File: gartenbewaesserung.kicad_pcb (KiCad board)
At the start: 2 copper layers, 57 x 73.5 mm, 13 parts, among them J1 24VDC IN, J2 Relais, J3 4..20mA Hydrostatischer Sensor, J4 1-Wire A, J5 1-Wire B, J6 ADS1115 Modul, Q1 IRLZ44N, U1 WeMos_D1_mini, U2 ULN2803A

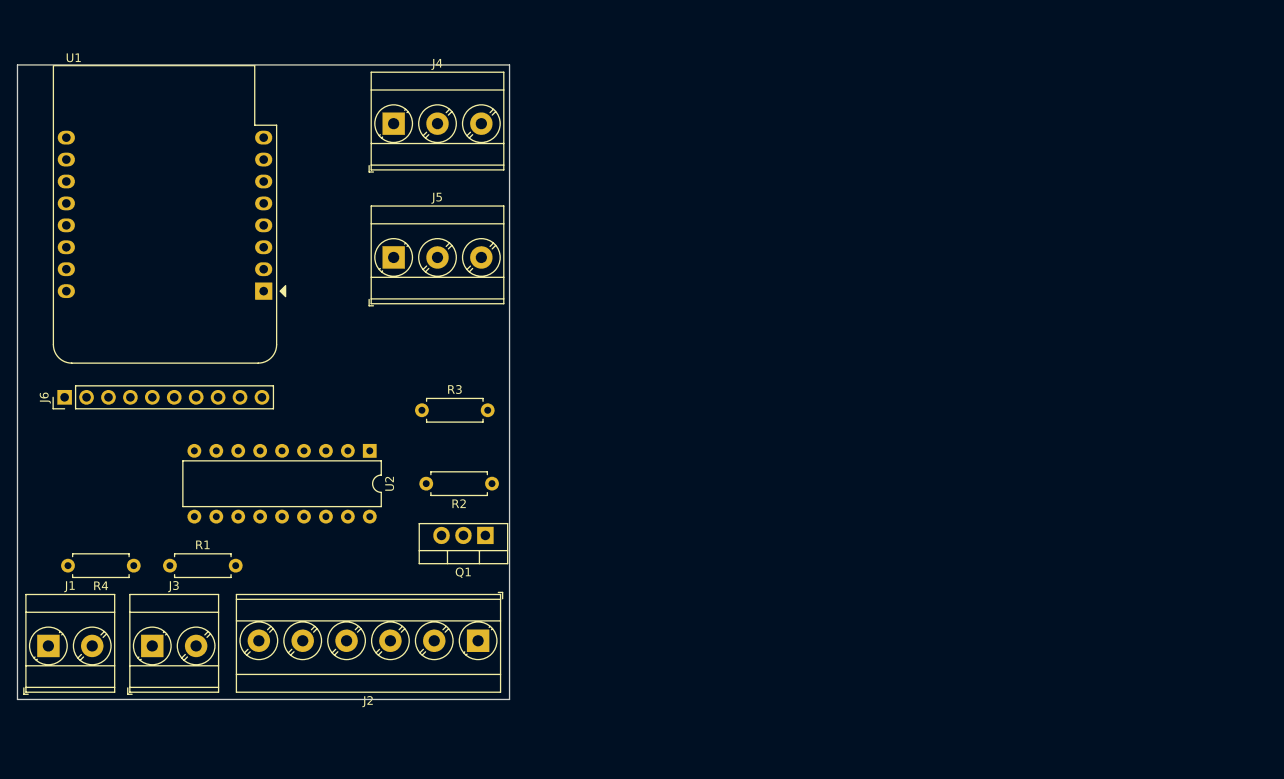
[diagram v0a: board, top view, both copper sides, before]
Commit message: Zustand bei Fertigstellung
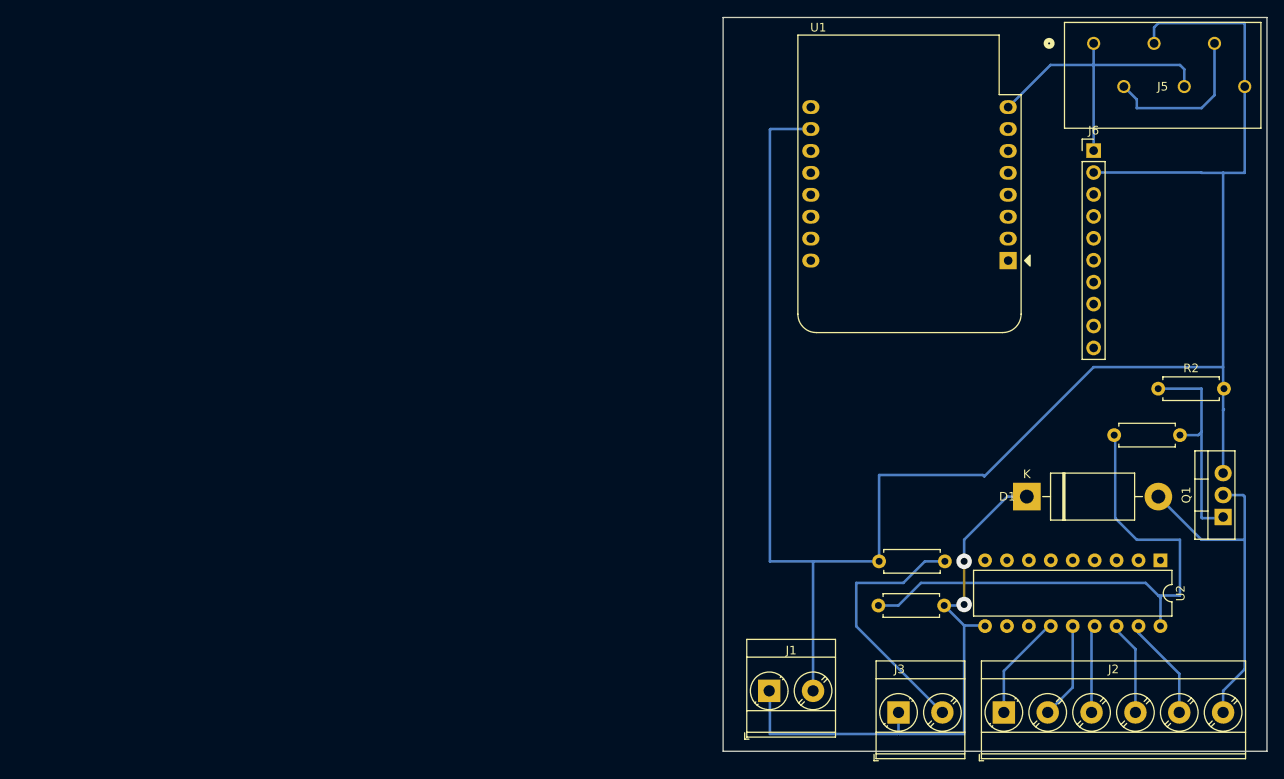
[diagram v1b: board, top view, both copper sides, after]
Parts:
- removed J4: 1-Wire A, TerminalBlock_Phoenix:TerminalBlock_Phoenix_MKDS-3-3-5.08_1x03_P5.08mm_Horizontal
- added D1: 1N5408, Diode_THT:D_DO-201AD_P15.24mm_Horizontal, F.Cu at (167.3, 97.5)
- J5: value 1-Wire B -> 250-206; footprint TerminalBlock_Phoenix:TerminalBlock_Phoenix_MKDS-3-3-5.08_1x03_P5.08mm_Horizontal -> footprints:CONN_250-206_WAG
- moved J6 122.6 mm to (175.0, 57.4), turned to 0 degrees
- moved R4 94.0 mm to (157.8, 105.0)
- moved U2 92.5 mm to (182.7, 104.9)
- moved R1 89.8 mm to (157.7, 110.1), turned to 180 degrees
- moved J3 86.8 mm to (152.4, 122.5)
- moved U1 86.3 mm to (165.1, 70.2)
- moved Q1 85.5 mm to (190.0, 99.9), turned to 90 degrees
- moved J5 84.8 mm to (175.0, 45.0)
- moved J1 83.7 mm to (137.4, 120.0)
- moved R3 80.2 mm to (177.4, 90.4)
- moved R2 77.9 mm to (182.5, 85.0), turned to 0 degrees
- moved J2 61.5 mm to (164.6, 122.5), turned to 0 degrees
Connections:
- J2 pad 6: Net-(J2-Pin_6) -> Net-(D1-A)
- J5 pad 2: Net-(J4-Pin_2) -> Net-(U1-D3)
- Q1 pad 2: Net-(J2-Pin_1) -> Net-(D1-A)
- U1 pad 12: Net-(J4-Pin_2) -> Net-(U1-D3)
- U1 pad 16: Net-(U1-TX) -> unconnected-(U1-TX-Pad16)
- U1 pad 3: unconnected-(U1-D0-Pad3) -> Net-(U1-D0)
- U2 pad 1: Net-(U1-TX) -> Net-(U1-D0)
- U2 pad 13: Net-(J2-Pin_6) -> Net-(J2-Pin_1)
- U2 pad 14: Net-(J2-Pin_5) -> Net-(J2-Pin_2)
- U2 pad 15: Net-(J2-Pin_4) -> Net-(J2-Pin_3)
- U2 pad 16: Net-(J2-Pin_3) -> Net-(J2-Pin_4)
- U2 pad 17: Net-(J2-Pin_2) -> Net-(J2-Pin_5)
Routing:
- net GND: track 0.00 -> 220.1 mm
- net +24V: track 0.00 -> 67.9 mm, vias 0 -> 2
- net Net-(U2-O1): track 0.00 -> 65.0 mm
- net Net-(D1-A): track 0.00 -> 40.7 mm
- net VCC: track 0.00 -> 37.0 mm
- net /A0: track 0.00 -> 30.4 mm
- net Net-(Q1-G): track 0.00 -> 25.6 mm
- net Net-(U1-D3): track 0.00 -> 18.7 mm
- net Net-(J2-Pin_1): track 0.00 -> 12.4 mm
- net Net-(J2-Pin_5): track 0.00 -> 12.0 mm
- net Net-(J2-Pin_2): track 0.00 -> 11.2 mm
- net Net-(J2-Pin_4): track 0.00 -> 10.9 mm
- net Net-(J2-Pin_3): track 0.00 -> 10.5 mm
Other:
- board size 57 x 73.5 mm -> 63 x 85 mm
